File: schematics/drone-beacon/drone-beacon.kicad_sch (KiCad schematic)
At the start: 13 parts, among them J1 ESP32 Flashing connector, J2 Power Input, SW1 Model selection, U1 ESP32-WROOM-32U, U2 AMS1117-3.3, U3 L80-R

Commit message: Update schematics
Signed-off-by: LAMBS Pierre-Antoine <pierreantoine.lambs@gmail.com>
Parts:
- J2: footprint (none) -> Connector_PinHeader_2.00mm:PinHeader_1x02_P2.00mm_Vertical
- U2: footprint Package_TO_SOT_SMD:SOT-89-3 -> Package_TO_SOT_SMD:SOT-223
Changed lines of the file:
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@@
 			)
 		)
-		(property "Footprint" "Package_TO_SOT_SMD:SOT-89-3"
+		(property "Footprint" "Package_TO_SOT_SMD:SOT-223"
 			(at 148.59 20.32 0)
 			(effects
@@
 			)
 		)
-		(property "Footprint" ""
+		(property "Footprint" "Connector_PinHeader_2.00mm:PinHeader_1x02_P2.00mm_Vertical"
 			(at 96.52 30.48 0)
 			(effects

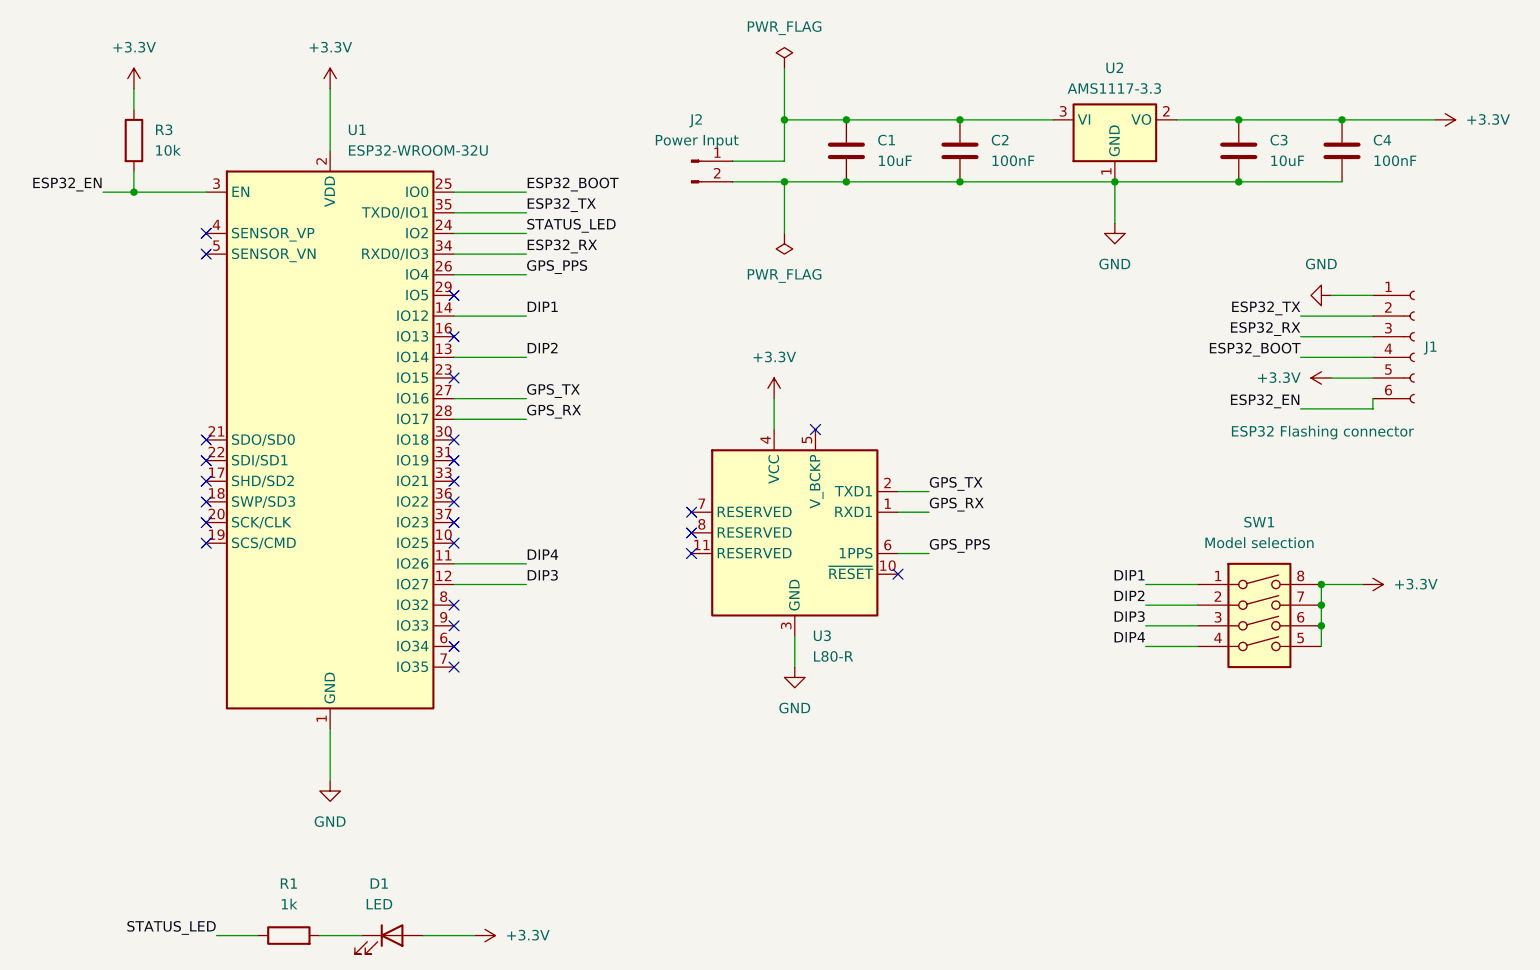
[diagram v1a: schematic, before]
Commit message: Update schematics
Signed-off-by: LAMBS Pierre-Antoine <pierreantoine.lambs@gmail.com>
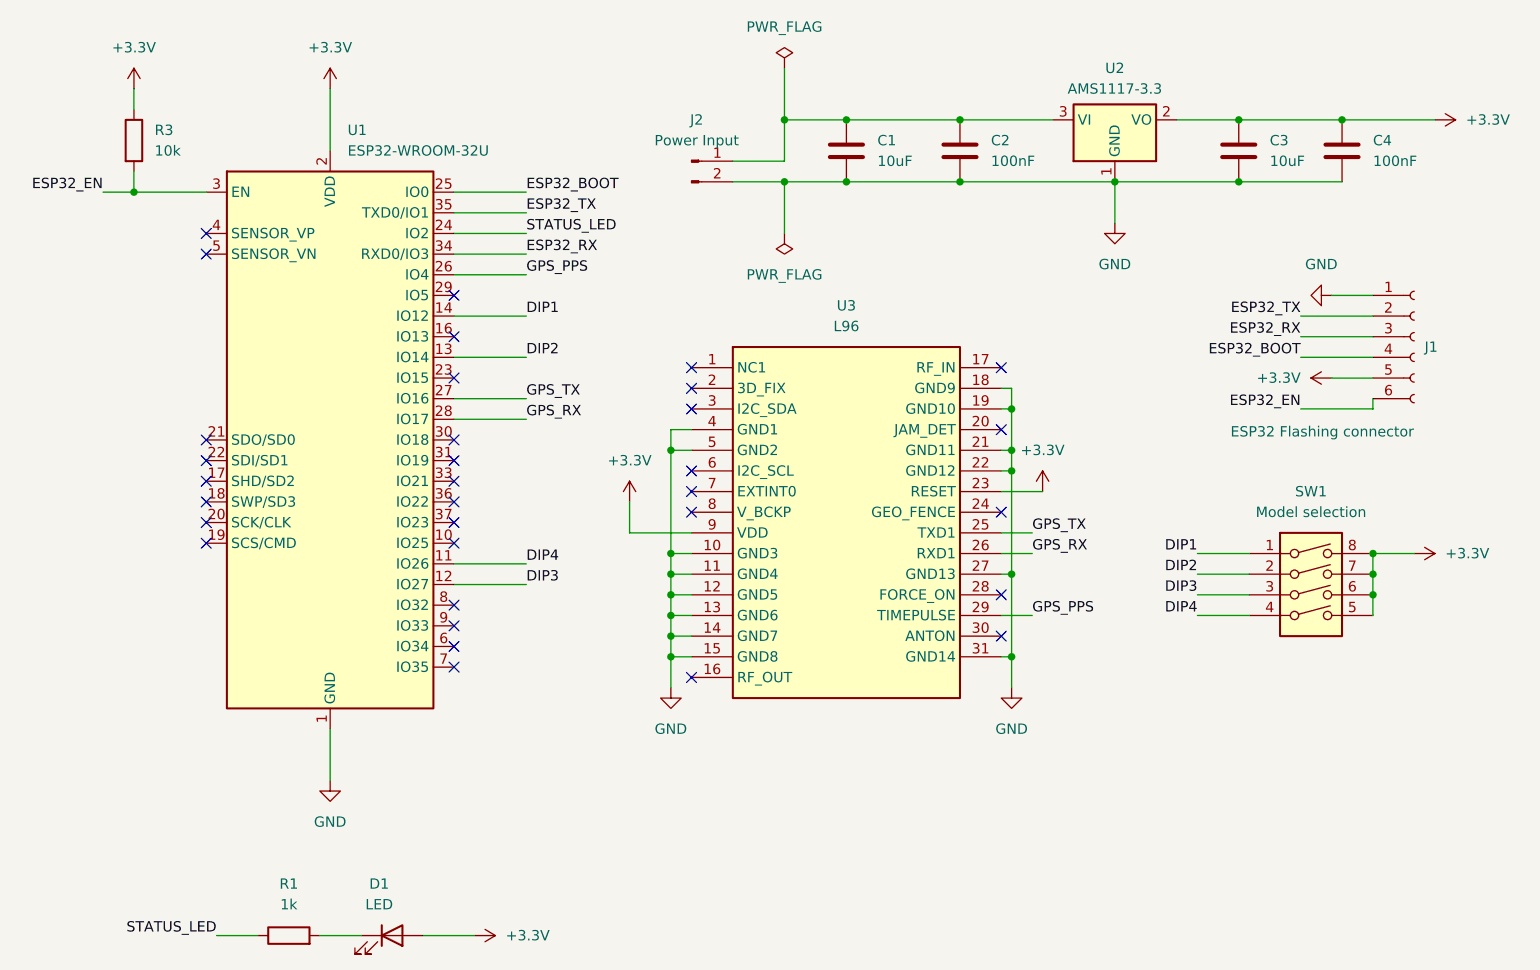
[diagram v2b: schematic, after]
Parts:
- C1, C2, C3, C4: footprint Capacitor_SMD:C_0201_0603Metric -> Capacitor_SMD:C_0402_1005Metric_Pad0.74x0.62mm_HandSolder
- D1: footprint LED_SMD:LED_0201_0603Metric -> LED_SMD:LED_0402_1005Metric_Pad0.77x0.64mm_HandSolder
- R1, R3: footprint Resistor_SMD:R_0201_0603Metric -> Resistor_SMD:R_0402_1005Metric_Pad0.72x0.64mm_HandSolder
- U3: value L80-R -> L96; footprint RF_GPS:Quectel_L96 -> QUECTEL_L96:L96; symbol RF_GPS:L80-R -> L96:L96-M33; Manufacturer_Name (none) -> Quectel; Manufacturer_Part_Number (none) -> L96-M33; Mouser Part Number (none) -> 277-L96-M33; Mouser Price/Stock (none) -> https://www.mouser.co.uk/ProductDetail/Quectel/L96-M33?qs=G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
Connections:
- net +3.3V: now also U3.23 (RESET), U3.9 (VDD); no longer U3.4 (VCC)
- net GND: now also U3.10 (GND3), U3.11 (GND4), U3.13 (GND6), U3.14 (GND7), U3.15 (GND8), U3.18 (GND9), U3.19 (GND10), U3.21 (GND11), U3.22 (GND12), U3.27 (GND13), U3.31 (GND14), U3.4 (GND1), U3.5 (GND2); no longer U3.3 (GND)
- net GPS_PPS: now also U3.29 (TIMEPULSE); no longer U3.6 (1PPS)
- net GPS_RX: now also U3.26 (RXD1); no longer U3.1 (RXD1)
- net GPS_TX: now also U3.25 (TXD1); no longer U3.2 (TXD1)
- no-connect marks 26 -> 33
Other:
- moved on the sheet: SW1
